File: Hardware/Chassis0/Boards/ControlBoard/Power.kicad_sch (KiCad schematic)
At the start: 51 parts

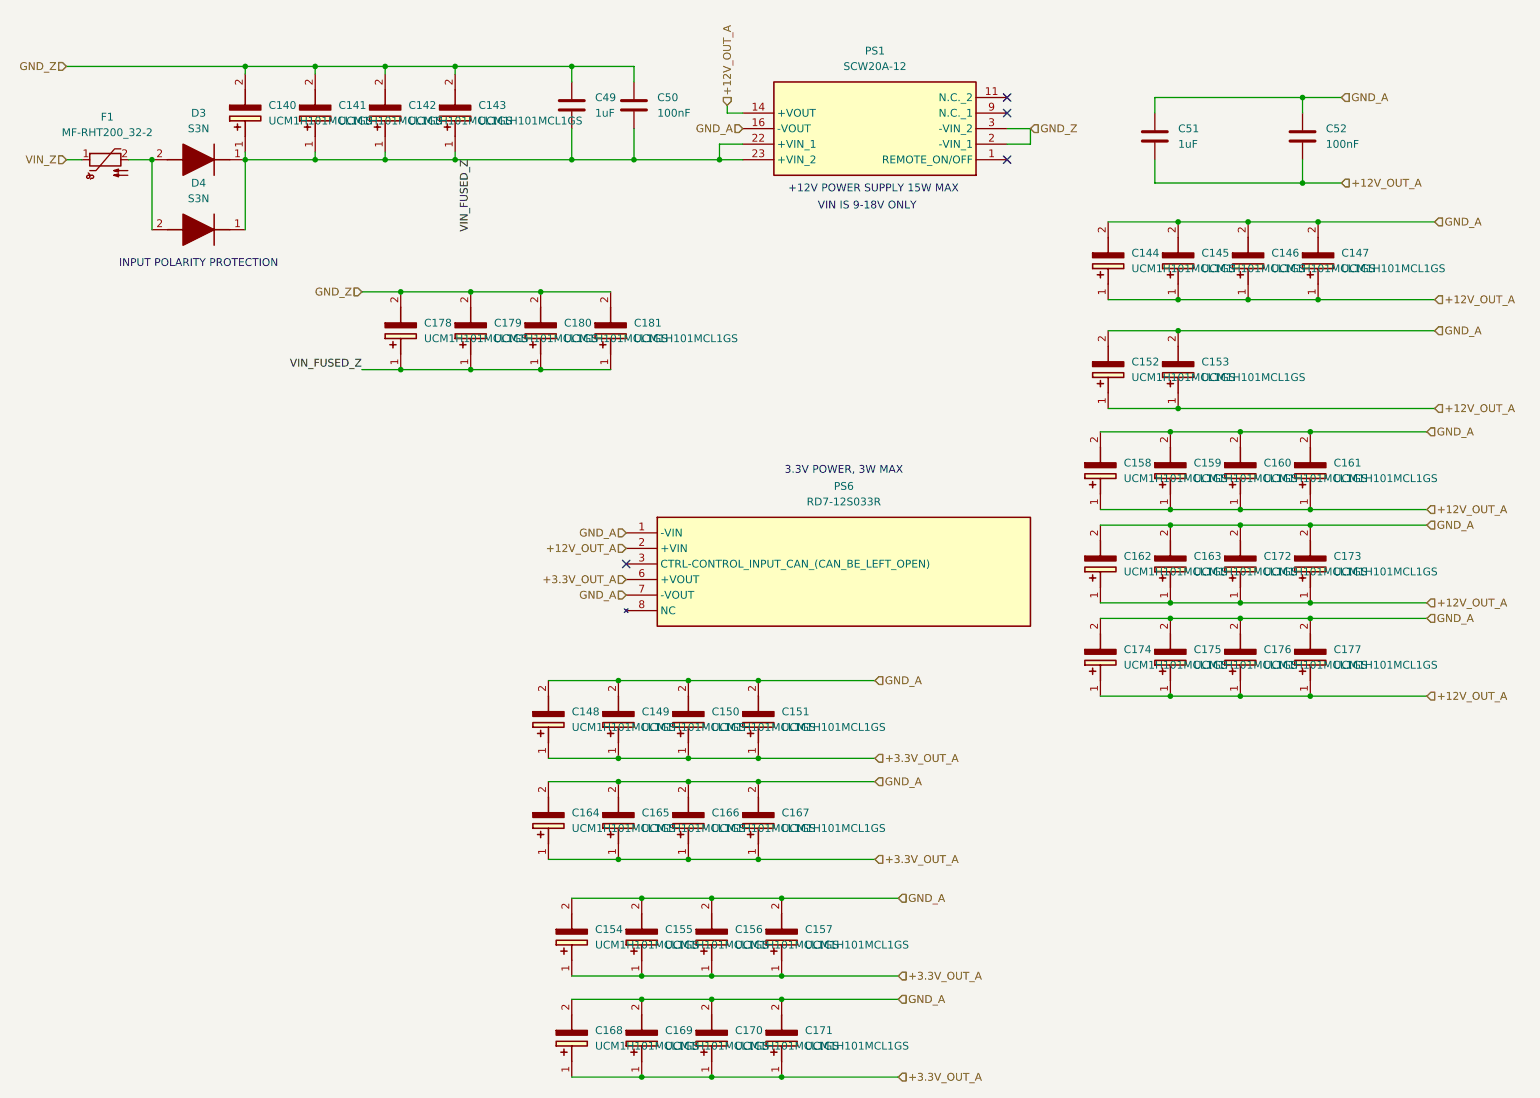
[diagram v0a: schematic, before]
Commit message: finish chassis 0 board design v1
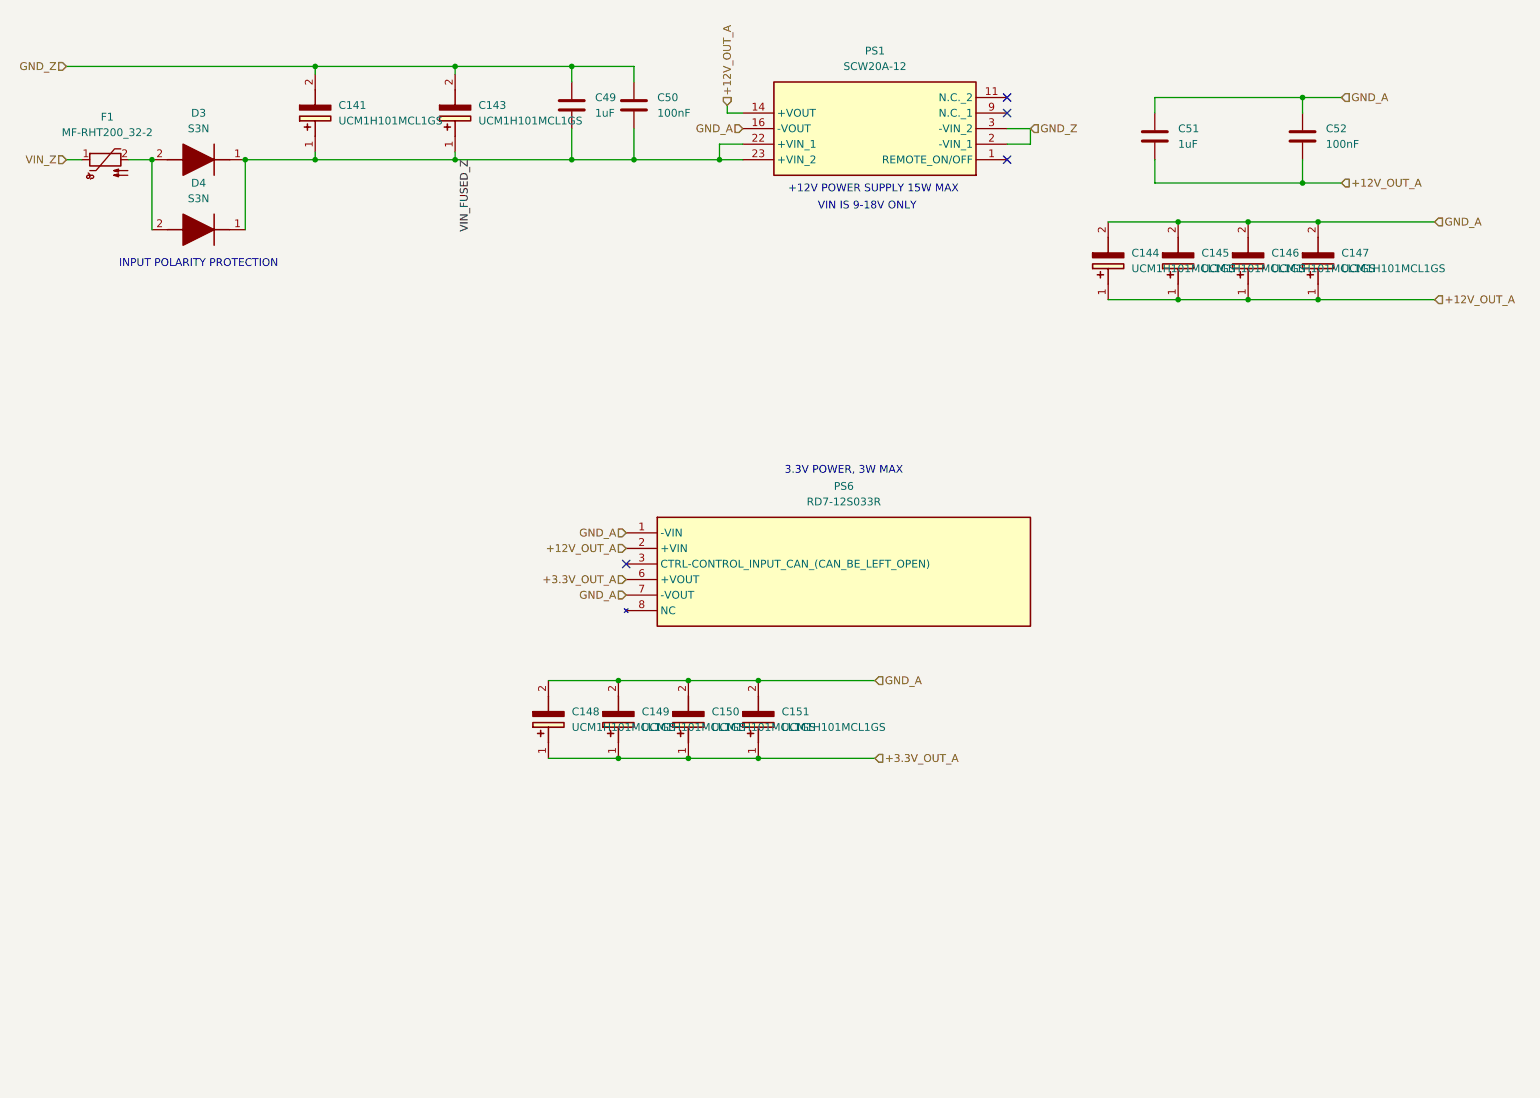
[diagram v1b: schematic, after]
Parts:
- removed C140, C142, C152, C153, C154, C155, C156, C157, C158, C159, C160, C161, C162, C163, C164, C165, C166, C167, C168, C169, C170, C171, C172, C173, C174, C175, C176, C177, C178, C179, C180, C181: UCM1H101MCL1GS, InverterCom:CAPAE660X800N, symbol InverterCom:UCM1H101MCL1GS
